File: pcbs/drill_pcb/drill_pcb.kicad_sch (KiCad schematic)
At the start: 30 parts, among them J1 24V IN, J10 DEEP WEIGHT SENSOR, J11 STEPPER STORAGE, J12 SURFACE WEIGHT SENSOR, J13 uC COMMUNICATION, J2 DC MOTOR 24 V, J3 DC MOTOR UART, J4 ENCODER VERTICAL DRIVE, J5 LIMIT SENSOR TOP, J6 HEIGHT SENSOR, J7 STEPPER VERTICAL DRIVE, J8 ENCODER STORAGE, J9 LIMIT SENSOR BOTTOM, U1 ESP32-DevKitC, U2 LM3940

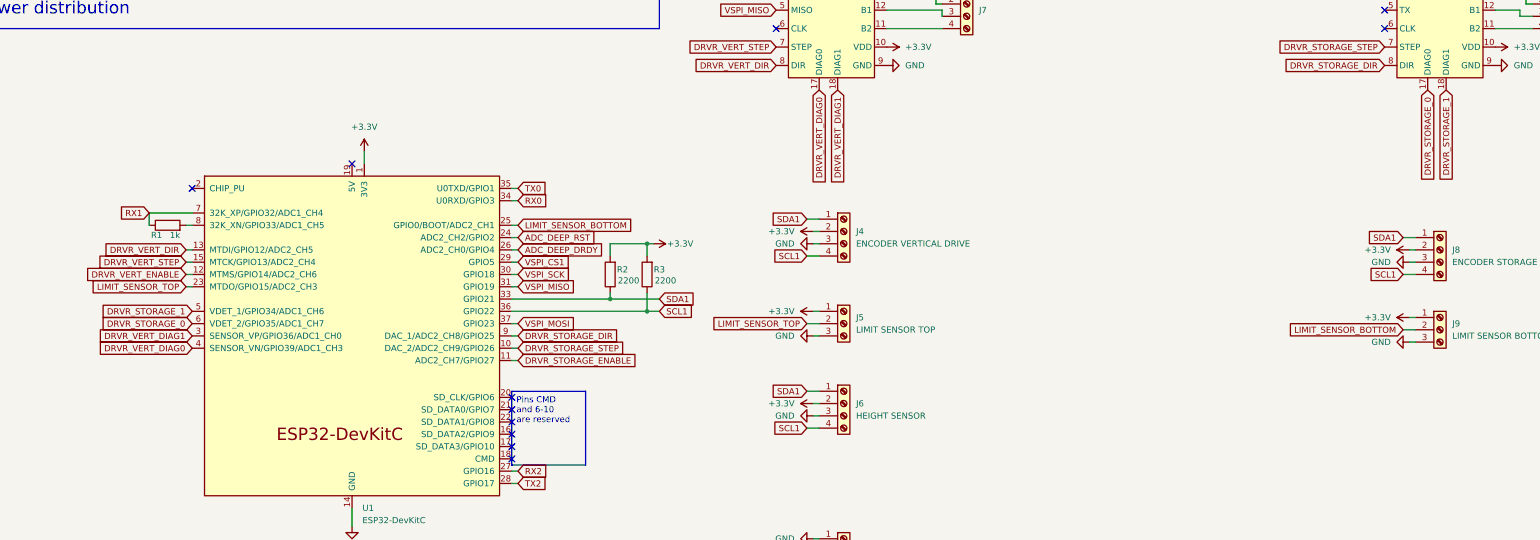
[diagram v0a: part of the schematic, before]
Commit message: pcb changes, code changes
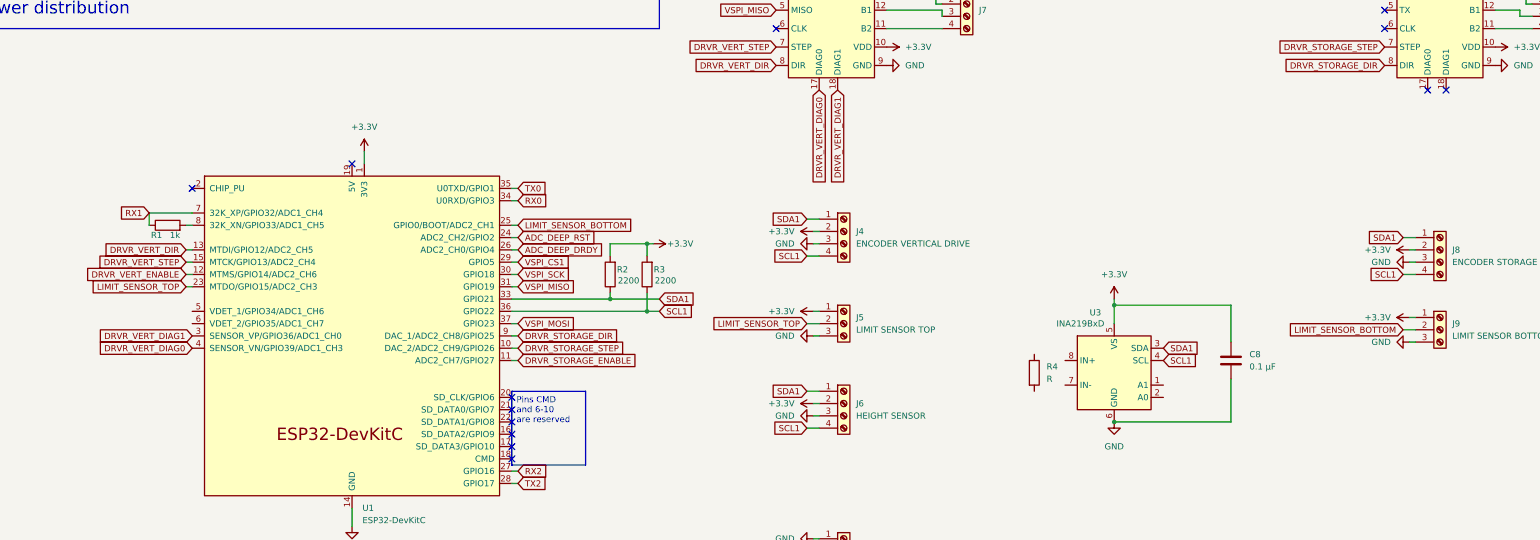
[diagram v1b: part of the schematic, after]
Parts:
- added C8: 0.1 μF, symbol Device:C
- added R4: R, symbol Device:R
- added U3: INA219BxD, Package_SO:SOIC-8_3.9x4.9mm_P1.27mm, symbol Sensor_Energy:INA219BxD
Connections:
- net +3.3V: now also C8.1, U3.5 (VS)
- net GND: now also C8.2, U3.6 (GND)
- net SCL1: now also U3.4 (SCL)
- net SDA1: now also U3.3 (SDA)
- net DRVR_STORAGE_0: no longer names the net of A2.17 (DIAG0)
- net DRVR_STORAGE_0: no longer U1.6 (VDET_2/GPIO35/ADC1_CH7)
- net DRVR_STORAGE_1: no longer names the net of A2.18 (DIAG1)
- net DRVR_STORAGE_1: no longer U1.5 (VDET_1/GPIO34/ADC1_CH6)
- no-connect marks 13 -> 15
